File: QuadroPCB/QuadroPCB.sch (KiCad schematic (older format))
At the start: 30 parts, among them IC1 AT24CS02-SSHM, P1 MPU9150, P10 AKKU, P11 led_power, P12 step_down, P13 leds1, P14 leds2, P2 stm32discovery_left, P3 stm32discovery_right, P4 rc_signal, P5 Motor3, P6 Motor4, P7 BMP180, P8 Motor1, P9 Motor2, Q1 Q_NMOS_GSD, Q2 Q_NMOS_GSD, U1 74HC595, U2 74HC595, U3 uln2803, U4 uln2803

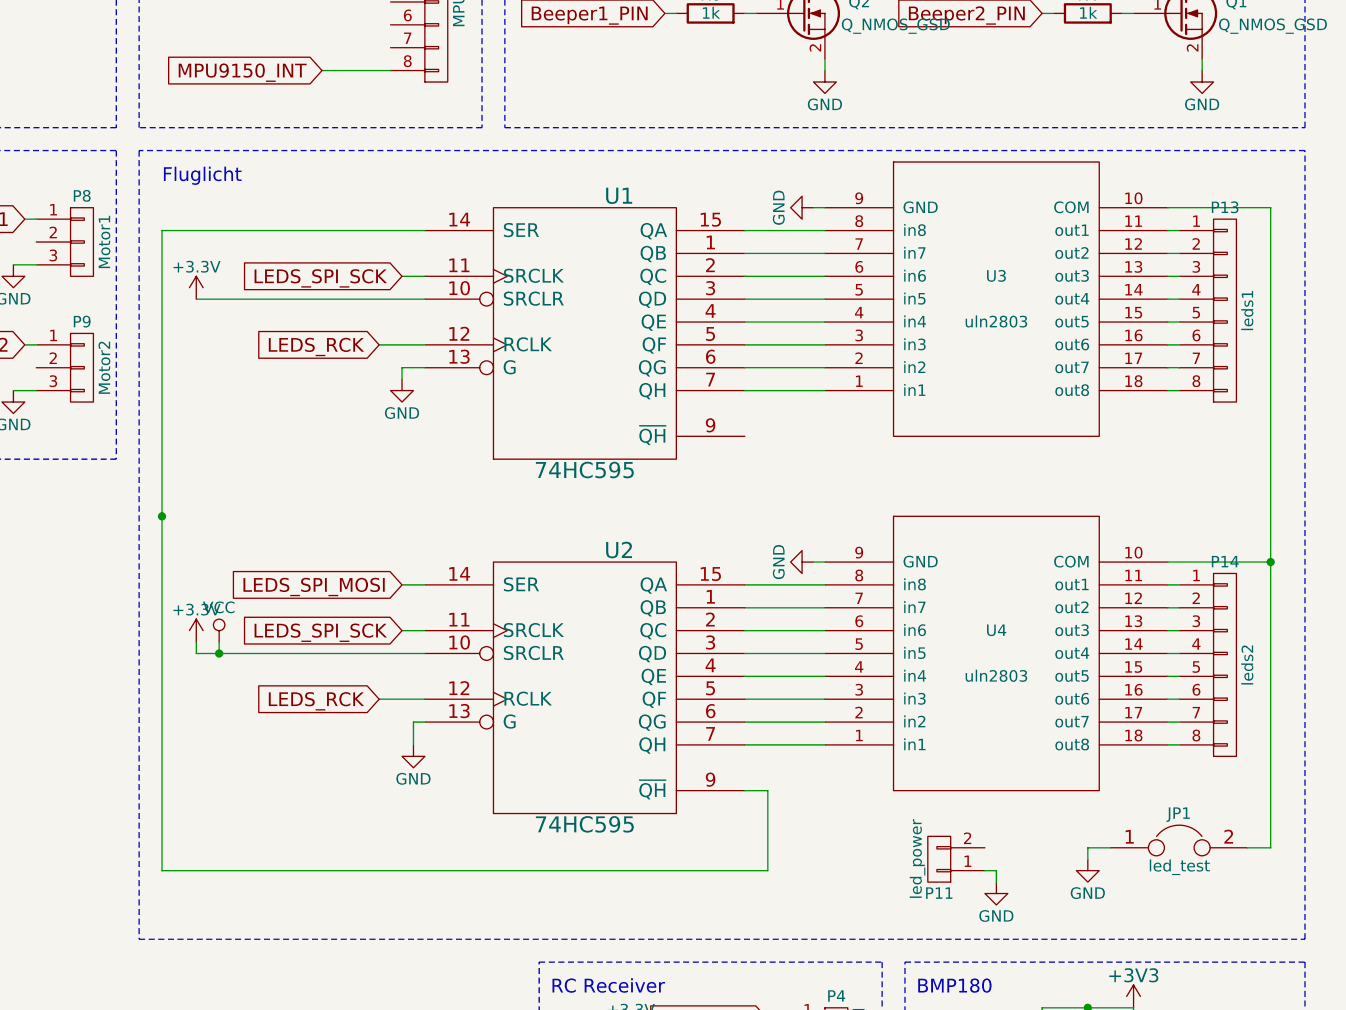
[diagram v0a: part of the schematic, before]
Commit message: version 1
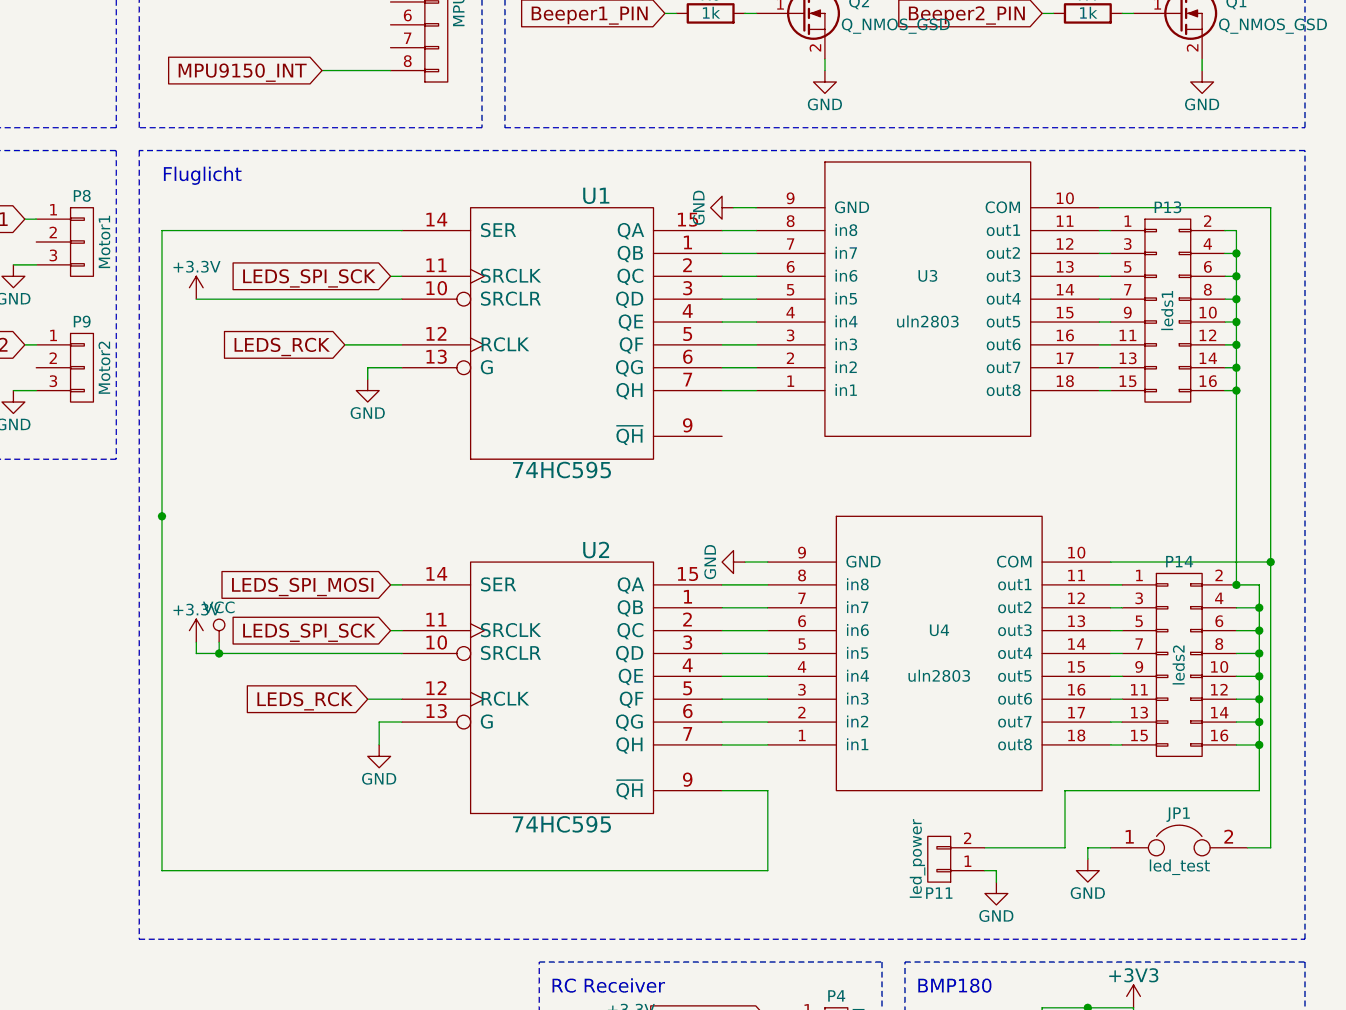
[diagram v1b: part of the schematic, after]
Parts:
- removed P13: leds1, Pin_Headers:Pin_Header_Straight_1x08, symbol CONN_01X08
- removed P14: leds2, Pin_Headers:Pin_Header_Straight_1x08, symbol CONN_01X08
- added P13: leds1, Pin_Headers:Pin_Header_Straight_2x08, symbol CONN_02X08
- added P14: leds2, Pin_Headers:Pin_Header_Straight_2x08, symbol CONN_02X08
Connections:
- net at U4.11 (out1): now also P14.1 (P1)
- net at U4.12 (out2): now also P14.3 (P3)
- net at U4.13 (out3): now also P14.5 (P5)
- net at U4.14 (out4): now also P14.7 (P7)
- net at U4.15 (out5): now also P14.9 (P9)
- net at U4.16 (out6): now also P14.11 (P11)
- net at U4.17 (out7): now also P14.13 (P13)
- net at U4.18 (out8): now also P14.15 (P15)
- net at U3.11 (out1): now also P13.1 (P1)
- net at U3.12 (out2): now also P13.3 (P3)
- net at U3.13 (out3): now also P13.5 (P5)
- net at U3.14 (out4): now also P13.7 (P7)
- net at U3.15 (out5): now also P13.9 (P9)
- net at U3.16 (out6): now also P13.11 (P11)
- net at U3.17 (out7): now also P13.13 (P13)
- net at U3.18 (out8): now also P13.15 (P15)
- net at P11.2 (P2): now also P13.10 (P10), P13.12 (P12), P13.14 (P14), P13.16 (P16), P13.2 (P2), P13.4 (P4), P13.6 (P6), P13.8 (P8), P14.10 (P10), P14.12 (P12), P14.14 (P14), P14.16 (P16), P14.2 (P2), P14.4 (P4), P14.6 (P6), P14.8 (P8)
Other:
- moved on the sheet: U1, U2, U3, U4
